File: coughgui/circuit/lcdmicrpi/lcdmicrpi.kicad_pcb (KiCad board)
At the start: 2 copper layers, 32.4 x 76.4 mm, 7 parts

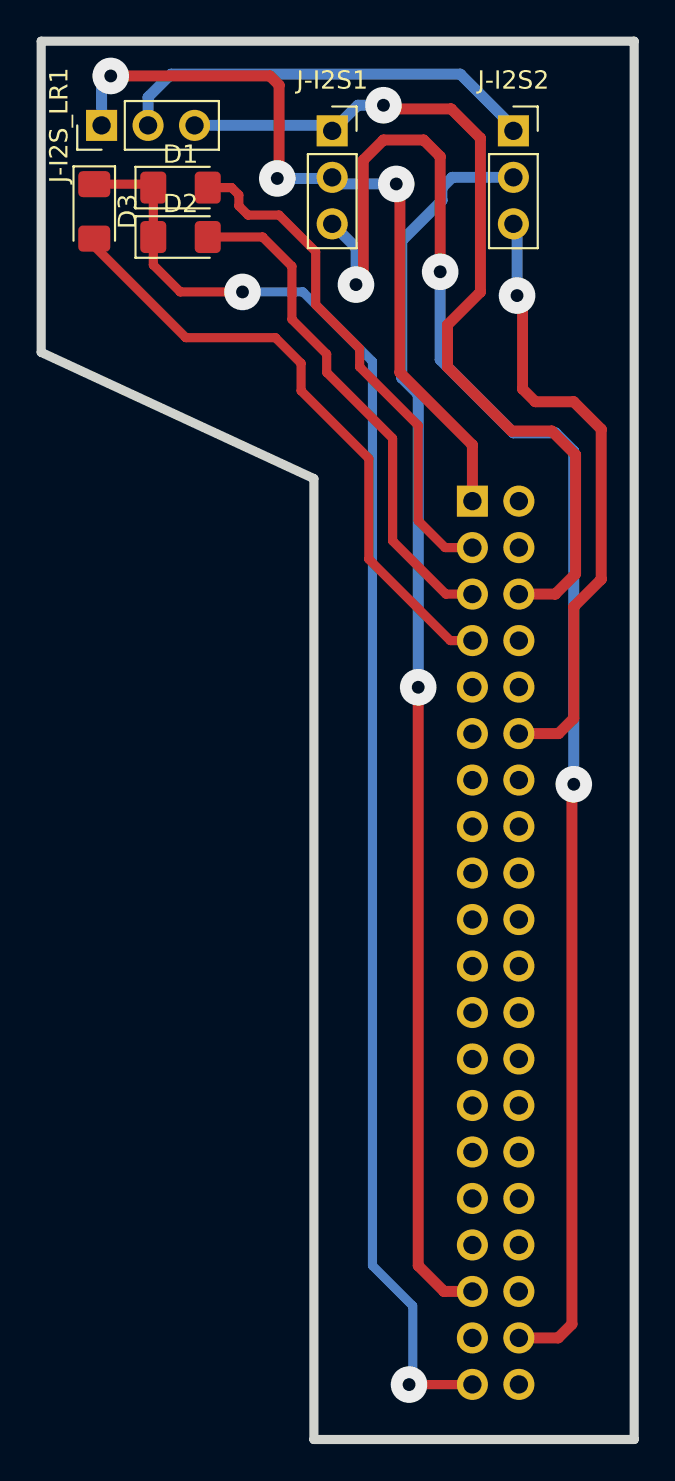
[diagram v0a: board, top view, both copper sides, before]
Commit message: pcb shield
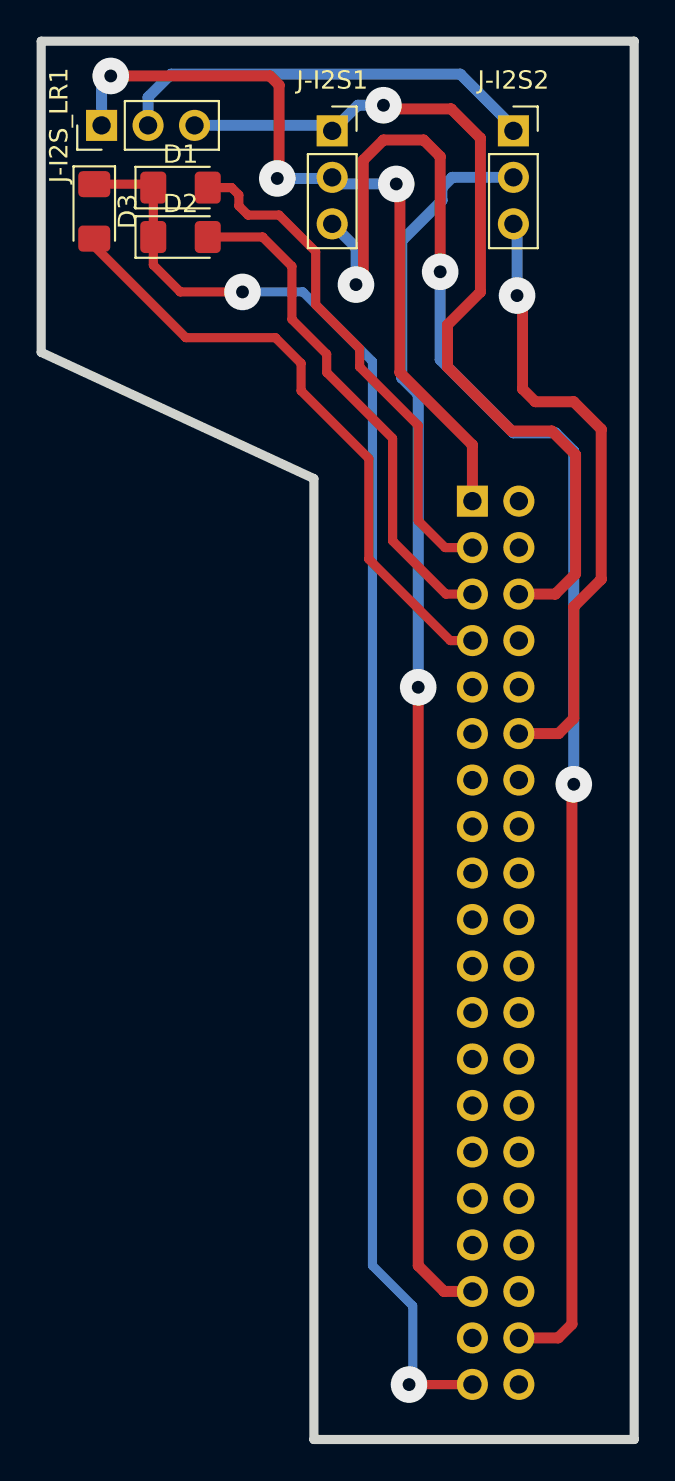
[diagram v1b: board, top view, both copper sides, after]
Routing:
- added copper zone on B.Cu, net (none)
- added copper zone on F.Cu, net (none)

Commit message: Project Stetoskop
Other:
- net class Default removed

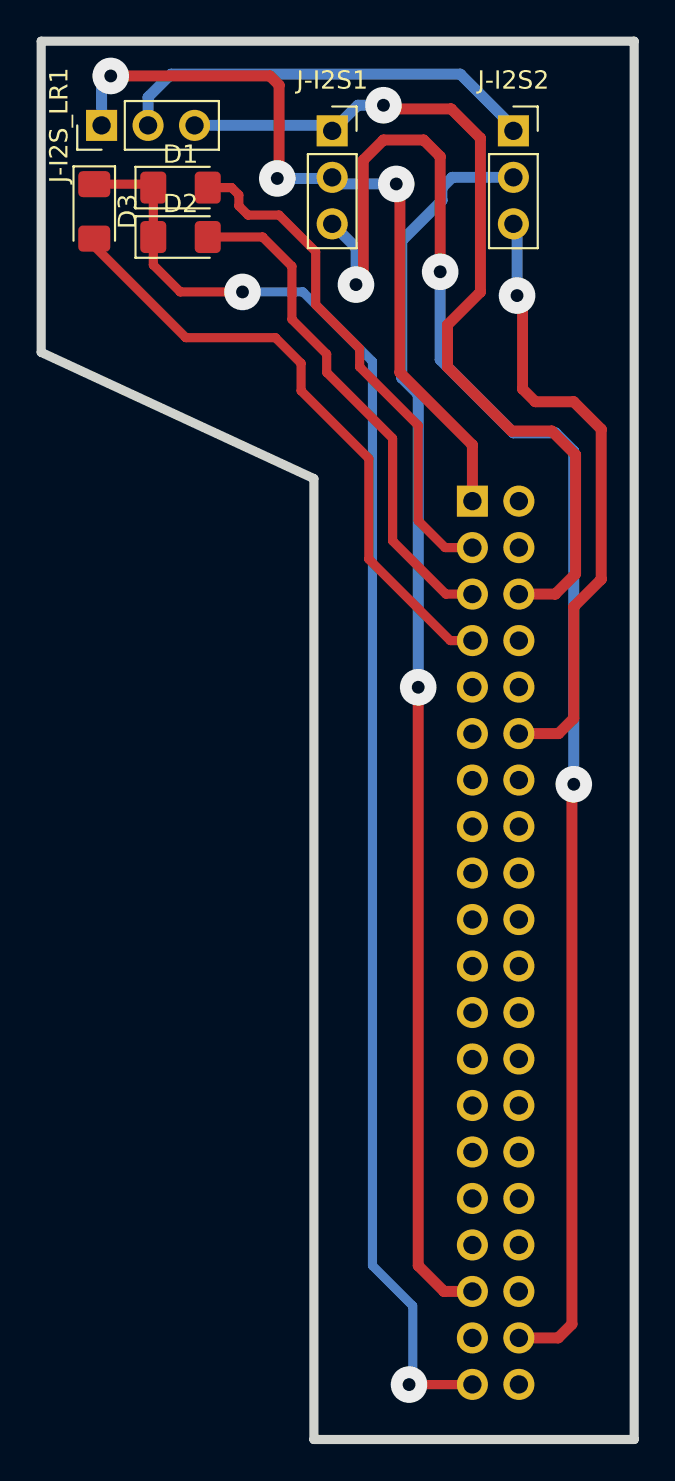
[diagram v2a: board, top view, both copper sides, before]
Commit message: some progress
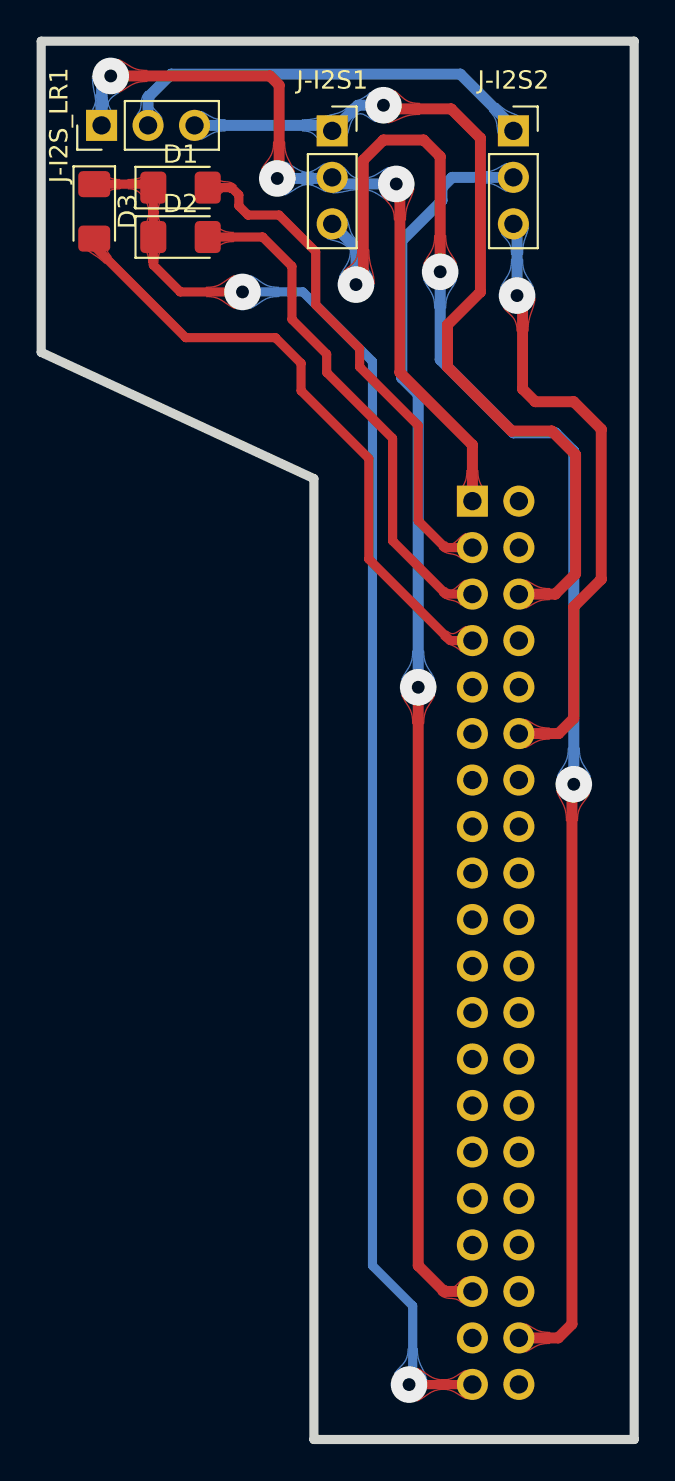
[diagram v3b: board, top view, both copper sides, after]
